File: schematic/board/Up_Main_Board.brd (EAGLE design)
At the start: 79.9 x 73.5 mm, 18 parts

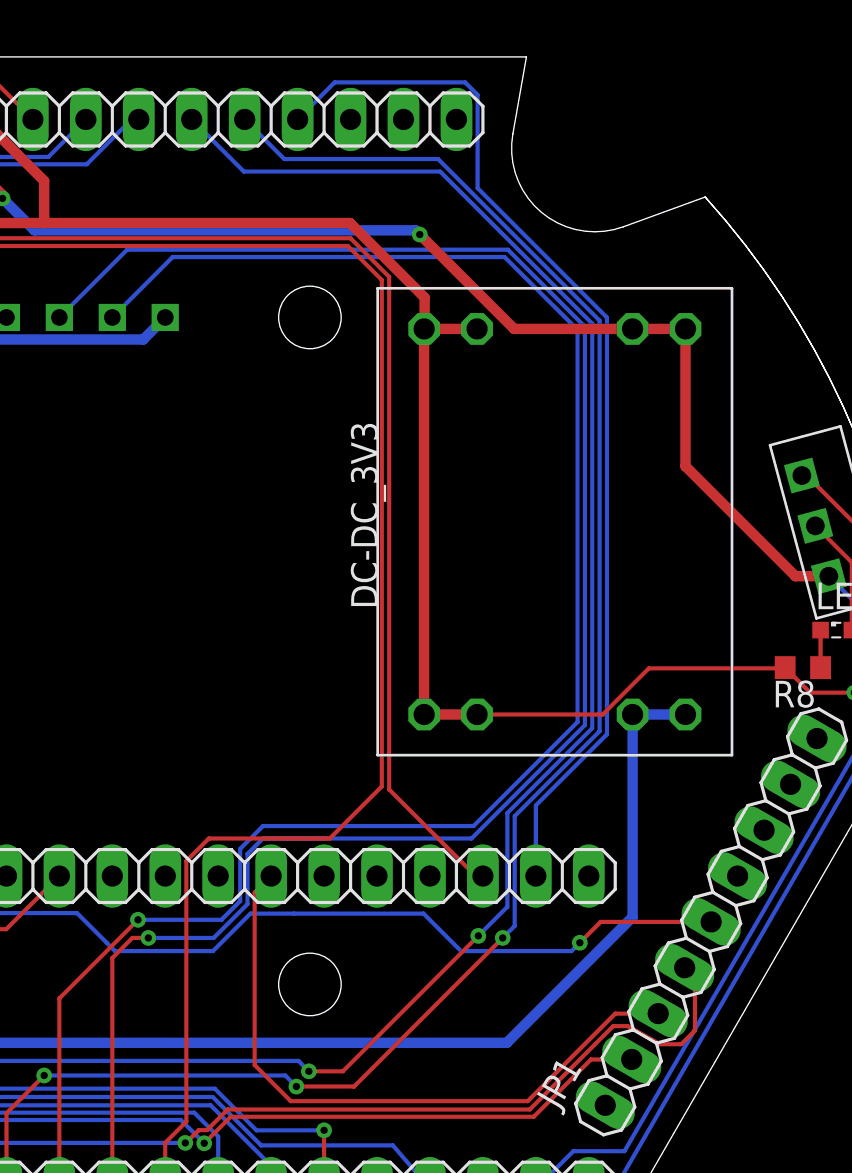
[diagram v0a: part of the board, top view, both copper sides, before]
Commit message: спонсор страданий
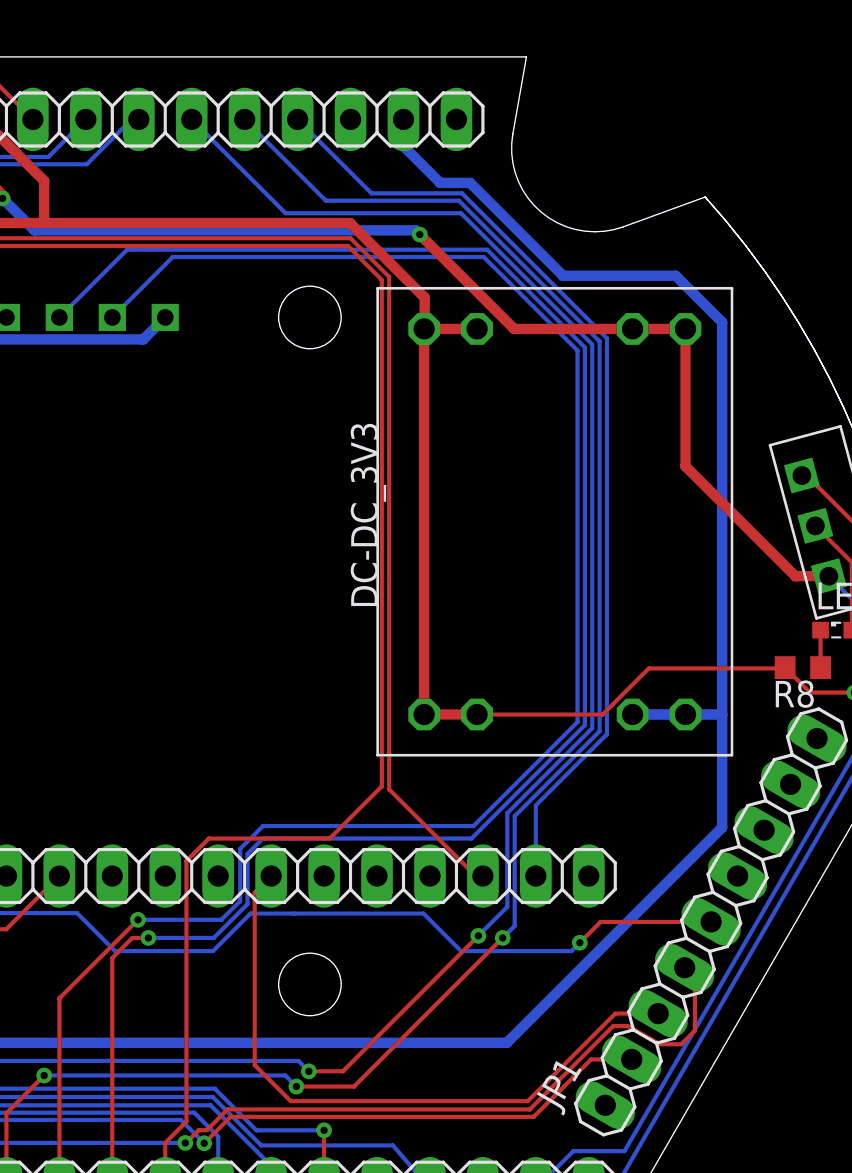
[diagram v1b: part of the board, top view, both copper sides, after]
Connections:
- removed net N$20: JP3.14
- net V_BAT: now also JP3.14
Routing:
- net V_BAT: track 118.4 -> 160.8 mm
- net CS_LSM: track 51.1 -> 46.4 mm
- net GPS_RX: track 87.0 -> 86.4 mm
- net 5MISO: track 83.9 -> 83.3 mm
- net 5MOSI: track 89.2 -> 88.6 mm
- net GPS_TX: track 84.7 -> 84.1 mm
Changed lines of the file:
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@@
 <wire x1="68.6" y1="46.6" x2="73.5904" y2="51.5904" width="0.2" layer="16"/>
 <wire x1="57.4044" y1="45.5044" x2="58.5" y2="46.6" width="0.2" layer="16"/>
-<wire x1="73.5904" y1="51.5904" x2="73.5904" y2="70.4096" width="0.2" layer="16"/>
-<wire x1="73.5904" y1="70.4096" x2="70.089884375" y2="73.8984125" width="0.2" layer="16"/>
+<wire x1="73.5904" y1="51.5904" x2="73.5904" y2="69.41294375" width="0.2" layer="16"/>
+<wire x1="73.5904" y1="69.41294375" x2="69.089884375" y2="73.8984125" width="0.2" layer="16"/>
 <wire x1="54.1684125" y1="73.8984125" x2="51.27" y2="71" width="0.2" layer="16"/>
-<wire x1="70.089884375" y1="73.8984125" x2="54.1684125" y2="73.8984125" width="0.2" layer="16"/>
+<wire x1="69.089884375" y1="73.8984125" x2="54.1684125" y2="73.8984125" width="0.2" layer="16"/>
 <wire x1="56.5044" y1="42.1" x2="57.4044" y2="43" width="0.2" layer="16"/>
 <wire x1="52.5" y1="42.1" x2="56.5044" y2="42.1" width="0.2" layer="16"/>
@@
 <wire x1="52.2306" y1="41.2306" x2="53" y2="41.2306" width="0.2" layer="1"/>
 <via x="53" y="41.2306" extent="1-16" drill="0.35"/>
-<wire x1="73.9428" y1="51.441175" x2="73.9428" y2="70.558825" width="0.2" layer="16"/>
-<wire x1="70.2508125" y1="74.2508125" x2="51.9808125" y2="74.2508125" width="0.2" layer="16"/>
+<wire x1="73.9428" y1="51.441175" x2="73.9428" y2="69.558825" width="0.2" layer="16"/>
+<wire x1="69.2508125" y1="74.2508125" x2="51.9808125" y2="74.2508125" width="0.2" layer="16"/>
 <wire x1="51.9808125" y1="74.2508125" x2="48.73" y2="71" width="0.2" layer="16"/>
-<wire x1="73.9428" y1="70.558825" x2="70.2508125" y2="74.2508125" width="0.2" layer="16"/>
+<wire x1="73.9428" y1="69.558825" x2="69.2508125" y2="74.2508125" width="0.2" layer="16"/>
 <wire x1="57.7568" y1="45.26338125" x2="58.49341875" y2="46" width="0.2" layer="16"/>
 <wire x1="57.7568" y1="42.854025" x2="57.7568" y2="45.26338125" width="0.2" layer="16"/>
@@
 <contactref element="U$2" pad="29"/>
 <contactref element="JP3" pad="11"/>
-<wire x1="57.62" y1="80.5" x2="59.52" y2="78.6" width="0.2" layer="16"/>
-<wire x1="59.52" y1="78.6" x2="66.901625" y2="78.6" width="0.2" layer="16"/>
-<wire x1="66.901625" y1="78.6" x2="74.6476" y2="70.854025" width="0.2" layer="16"/>
-<wire x1="74.6476" y1="70.854025" x2="74.6476" y2="51.145975" width="0.2" layer="16"/>
+<wire x1="57.62" y1="80.5" x2="61.52" y2="76.6" width="0.2" layer="16"/>
+<wire x1="61.52" y1="76.6" x2="67.901625" y2="76.6" width="0.2" layer="16"/>
+<wire x1="67.901625" y1="76.6" x2="74.6476" y2="69.854025" width="0.2" layer="16"/>
+<wire x1="74.6476" y1="69.854025" x2="74.6476" y2="51.145975" width="0.2" layer="16"/>
 <wire x1="74.6476" y1="51.145975" x2="70.5756" y2="47.073975" width="0.2" layer="16"/>
 <wire x1="70.5756" y1="41.8062" x2="70" y2="41.2306" width="0.2" layer="16"/>
@@
 <contactref element="U$2" pad="27"/>
 <contactref element="JP3" pad="10"/>
-<wire x1="55.08" y1="80.5" x2="57.58" y2="78" width="0.2" layer="16"/>
-<wire x1="57.58" y1="78" x2="67" y2="78" width="0.2" layer="16"/>
-<wire x1="67" y1="78" x2="74.2952" y2="70.7048" width="0.2" layer="16"/>
-<wire x1="74.2952" y1="70.7048" x2="74.2952" y2="51.2952" width="0.2" layer="16"/>
+<wire x1="55.08" y1="80.5" x2="59.58" y2="76" width="0.2" layer="16"/>
+<wire x1="59.58" y1="76" x2="68" y2="76" width="0.2" layer="16"/>
+<wire x1="68" y1="76" x2="74.2952" y2="69.7048" width="0.2" layer="16"/>
+<wire x1="74.2952" y1="69.7048" x2="74.2952" y2="51.2952" width="0.2" layer="16"/>
 <wire x1="74.2952" y1="51.2952" x2="70.2232" y2="47.2232" width="0.2" layer="16"/>
 <wire x1="70.2232" y1="47.2232" x2="70.2232" y2="42.7232" width="0.2" layer="16"/>
@@
 <wire x1="71.59" y1="44.2" x2="71.59" y2="47.59" width="0.2" layer="16"/>
 <wire x1="71.59" y1="47.59" x2="75" y2="51" width="0.2" layer="16"/>
-<wire x1="75" y1="51" x2="75" y2="71" width="0.2" layer="16"/>
-<wire x1="68.7944" y1="81.68218125" x2="68.20018125" y2="82.2764" width="0.2" layer="16"/>
-<wire x1="68.7944" y1="77.2056" x2="68.7944" y2="81.68218125" width="0.2" layer="16"/>
-<wire x1="61.9364" y1="82.2764" x2="60.16" y2="80.5" width="0.2" layer="16"/>
-<wire x1="75" y1="71" x2="68.7944" y2="77.2056" width="0.2" layer="16"/>
-<wire x1="68.20018125" y1="82.2764" x2="61.9364" y2="82.2764" width="0.2" layer="16"/>
+<wire x1="75" y1="70" x2="75" y2="51" width="0.2" layer="16"/>
+<wire x1="60.16" y1="80.5" x2="63.7076" y2="76.9524" width="0.2" layer="16"/>
+<wire x1="63.7076" y1="76.9524" x2="68.0476" y2="76.9524" width="0.2" layer="16"/>
+<wire x1="68.0476" y1="76.9524" x2="75" y2="70" width="0.2" layer="16"/>
 </signal>
 <signal name="5V">
@@
 <wire x1="46.4344" y1="21.5656" x2="46.4344" y2="26.2443125" width="0.5" layer="1"/>
 <wire x1="46.4344" y1="26.2443125" x2="45.6051125" y2="27.0736" width="0.5" layer="1"/>
-<wire x1="76.23" y1="51.95" x2="78.77" y2="51.95" width="0.5" layer="16"/>
-<wire x1="76.23" y1="42.23" x2="70.2" y2="36.2" width="0.5" layer="16"/>
-<wire x1="76.23" y1="42.23" x2="76.23" y2="51.95" width="0.5" layer="16"/>
+<wire x1="80.53" y1="46.53" x2="70.2" y2="36.2" width="0.5" layer="16"/>
 <wire x1="45.6051125" y1="27.0736" x2="32.9964875" y2="27.0736" width="0.5" layer="1"/>
 <wire x1="32.9964875" y1="27.0736" x2="32.2144" y2="27.8556875" width="0.5" layer="1"/>
@@
 <wire x1="29.63" y1="50.35" x2="29.63" y2="42.5844" width="0.5" layer="1"/>
 <wire x1="32.2144" y1="40" x2="29.63" y2="42.5844" width="0.5" layer="1"/>
+<contactref element="JP3" pad="14"/>
+<wire x1="80.53" y1="46.53" x2="80.53" y2="51.95" width="0.5" layer="16"/>
+<wire x1="80.53" y1="51.95" x2="80.53" y2="70.77" width="0.5" layer="16"/>
+<wire x1="80.53" y1="70.77" x2="78.3" y2="73" width="0.5" layer="16"/>
+<wire x1="72.89180625" y1="73" x2="78.3" y2="73" width="0.5" layer="16"/>
+<wire x1="65.24" y1="80.5" x2="65.24" y2="79.2148" width="0.5" layer="16"/>
+<wire x1="65.24" y1="79.2148" x2="67" y2="77.4548" width="0.5" layer="16"/>
+<wire x1="67" y1="77.4548" x2="68.43700625" y2="77.4548" width="0.5" layer="16"/>
+<wire x1="68.43700625" y1="77.4548" x2="72.89180625" y2="73" width="0.5" layer="16"/>
+<wire x1="76.23" y1="51.95" x2="78.77" y2="51.95" width="0.5" layer="16"/>
+<wire x1="78.77" y1="51.95" x2="78.82" y2="51.95" width="0.5" layer="16"/>
+<wire x1="78.82" y1="51.95" x2="80.53" y2="51.95" width="0.5" layer="16"/>
 </signal>
 <signal name="PHOTORES">
@@
 <contactref element="JP3" pad="13"/>
 </signal>
-<signal name="N$20">
-<contactref element="JP3" pad="14"/>
-</signal>
 <signal name="N$21">
